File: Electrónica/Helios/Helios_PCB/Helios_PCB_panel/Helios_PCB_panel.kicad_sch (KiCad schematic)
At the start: 46 parts, among them M0_0 Conn_01x04_Pin, M0_1 Conn_01x04_Pin, M0_2 Conn_01x04_Pin, M0_3 Conn_01x04_Pin, M1_0 Conn_01x04_Pin, M1_1 Conn_01x04_Pin, M1_2 Conn_01x04_Pin, M1_3 Conn_01x04_Pin, M2_0 Conn_01x04_Pin, M2_1 Conn_01x04_Pin, M2_2 Conn_01x04_Pin, M2_3 Conn_01x04_Pin, SW1 SW_SPDT

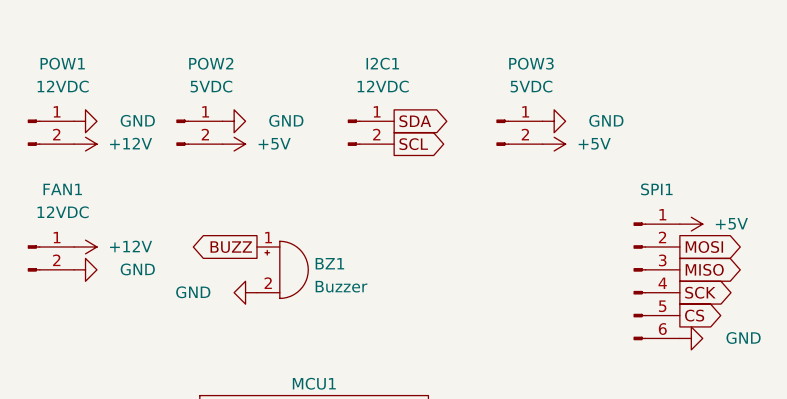
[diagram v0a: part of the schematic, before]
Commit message: PCBs ready for manufacturing
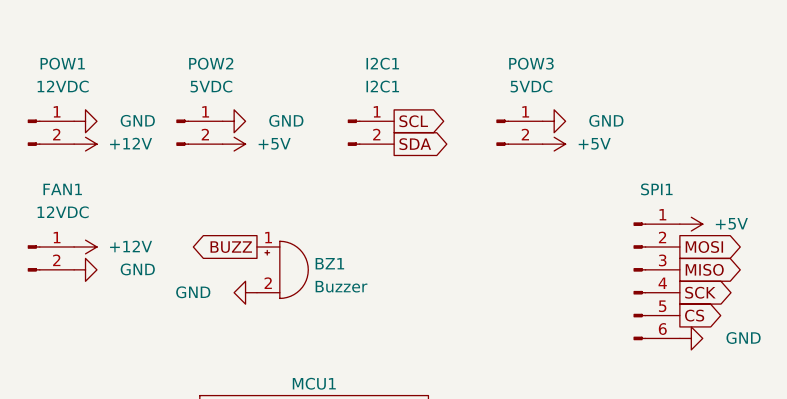
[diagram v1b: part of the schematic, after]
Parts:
- I2C1: value 12VDC -> I2C1
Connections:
- net SCL: now also I2C1.1 (Pin_1); no longer I2C1.2 (Pin_2)
- net SDA: now also I2C1.2 (Pin_2); no longer I2C1.1 (Pin_1)
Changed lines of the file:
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@@
-    )
-  )
-  (global_label "SCL" (shape output) (at 236.22 30.48 0) (fields_autoplaced)
-    (effects (font (size 1.27 1.27)) (justify left))
-    (property "Intersheetrefs" "${INTERSHEET_REFS}" (at 242.6334 30.48 0)
-      (effects (font (size 1.27 1.27)) (justify left) hide)
     )
   )
@@
     )
   )
+  (global_label "SCL" (shape output) (at 236.22 27.94 0) (fields_autoplaced)
+    (effects (font (size 1.27 1.27)) (justify left))
+    (property "Intersheetrefs" "${INTERSHEET_REFS}" (at 242.6334 27.94 0)
+      (effects (font (size 1.27 1.27)) (justify left) hide)
+    )
+  )
   (global_label "EN1" (shape input) (at 24.13 85.09 180) (fields_autoplaced)
     (effects (font (size 1.27 1.27)) (justify right))
@@
     )
   )
+  (global_label "SDA" (shape output) (at 236.22 30.48 0) (fields_autoplaced)
+    (effects (font (size 1.27 1.27)) (justify left))
+    (property "Intersheetrefs" "${INTERSHEET_REFS}" (at 242.6939 30.48 0)
+      (effects (font (size 1.27 1.27)) (justify left) hide)
+    )
+  )
   (global_label "EN2" (shape input) (at 209.55 85.09 180) (fields_autoplaced)
     (effects (font (size 1.27 1.27)) (justify right))
@@
     (property "Intersheetrefs" "${INTERSHEET_REFS}" (at 204.2252 92.71 0)
       (effects (font (size 1.27 1.27)) (justify right) hide)
-    )
-  )
-  (global_label "SDA" (shape output) (at 236.22 27.94 0) (fields_autoplaced)
-    (effects (font (size 1.27 1.27)) (justify left))
-    (property "Intersheetrefs" "${INTERSHEET_REFS}" (at 242.6939 27.94 0)
-      (effects (font (size 1.27 1.27)) (justify left) hide)
     )
   )
@@
     (pin "19")
     (pin "2")
+    (pin "20")
+    (pin "21")
+    (pin "22")
+    (pin "23")
+    (pin "24")
+    (pin "25")
+    (pin "26")
+    (pin "27")
+    (pin "28")
+    (pin "29")
+    (pin "3")
+    (pin "30")
+    (pin "31")
+    (pin "32")
+    (pin "33")
+    (pin "34")
+    (pin "35")
+    (pin "36")
+    (pin "37")
     (pin "38")
-    (pin "37")
-    (pin "36")
-    (pin "35")
-    (pin "34")
-    (pin "33")
-    (pin "32")
-    (pin "31")
-    (pin "30")
-    (pin "29")
-    (pin "3")
-    (pin "28")
-    (pin "27")
-    (pin "26")
-    (pin "25")
-    (pin "24")
-    (pin "23")
-    (pin "22")
-    (pin "21")
-    (pin "20")
     (pin "4")
     (pin "5")
@@
       (effects (font (size 1.27 1.27)))
     )
-    (property "Value" "12VDC" (at 234.95 24.13 0)
-      (effects (font (size 1.27 1.27)))
-    )
+    (property "Value" "I2C1" (at 234.95 24.13 0)
+      (effects (font (size 1.27 1.27)))
+    )
